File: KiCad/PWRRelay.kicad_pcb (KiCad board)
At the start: 2 copper layers, 46.4 x 65.4 mm, 19 parts, among them J0 Conn_01x02, K1 SANYOU_SRD_Form_C, Q1 IRLML2060, Q2 IRLML2060, U1 MOC3063M, X2 Conn_01x03_Male

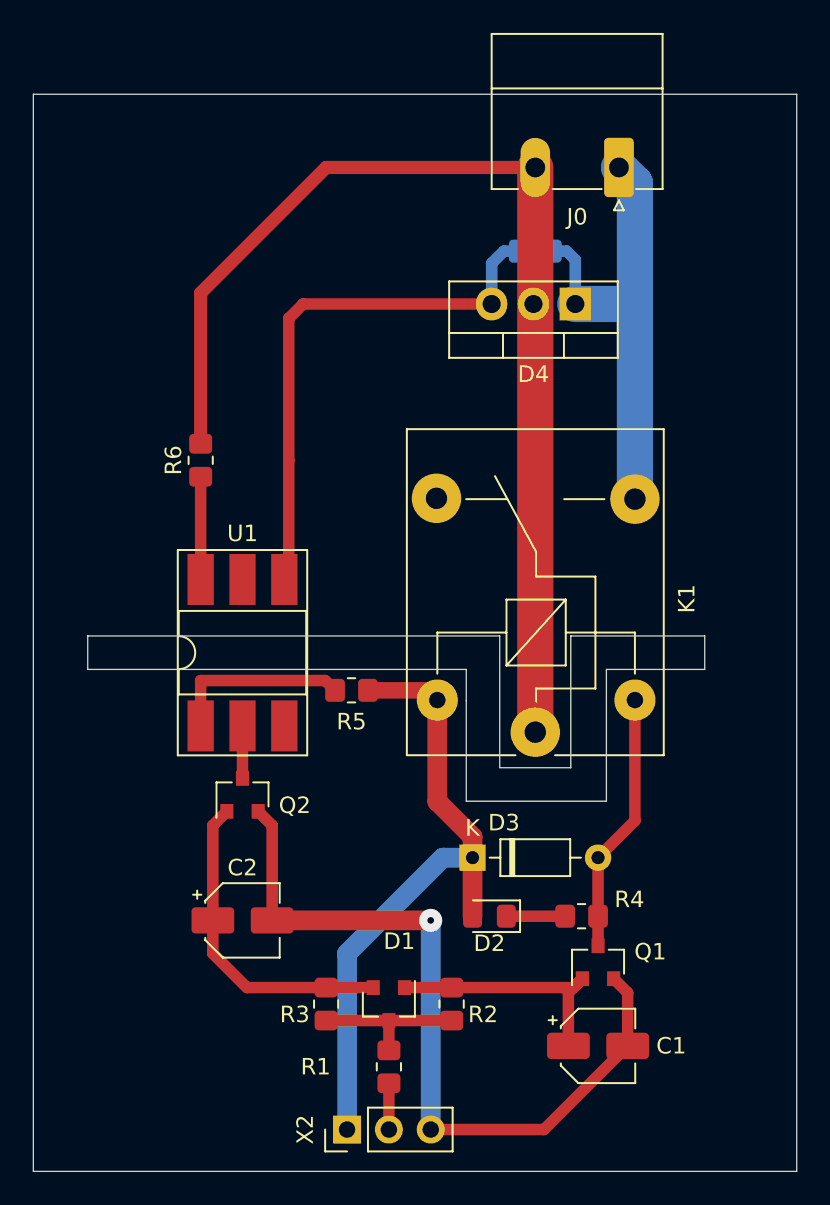
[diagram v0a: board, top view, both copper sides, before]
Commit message: Rework
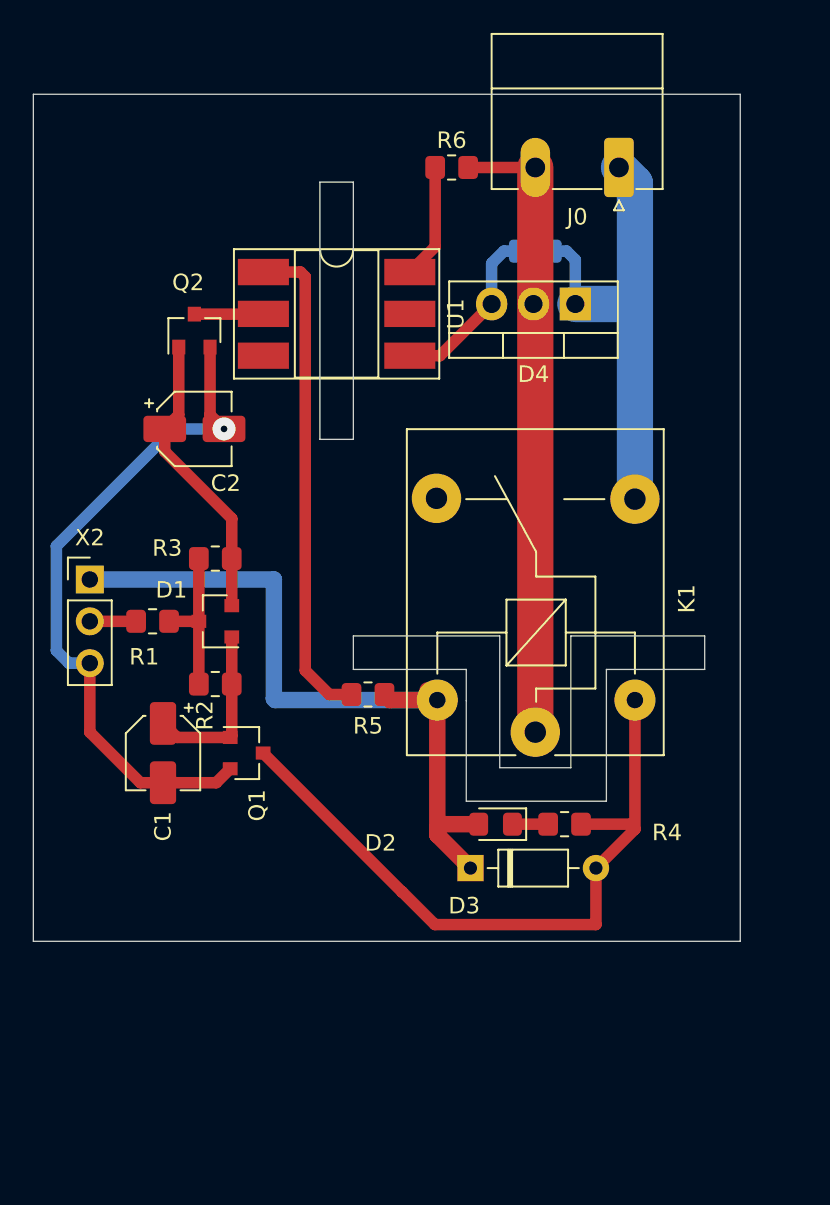
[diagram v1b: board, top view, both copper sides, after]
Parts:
- moved X2 36.9 mm to (33.9, 54.2), turned to 0 degrees
- moved C1 31.8 mm to (38.4, 64.8), turned to 270 degrees
- moved R1 30.6 mm to (37.7, 56.8), turned to 0 degrees
- moved C2 30.0 mm to (40.3, 45.1)
- moved Q2 28.3 mm to (40.3, 39.1)
- moved R3 27.9 mm to (41.5, 53.0), turned to 0 degrees
- moved D1 25.5 mm to (41.5, 56.8), turned to 180 degrees
- moved Q1 24.8 mm to (43.4, 64.8), turned to 0 degrees
- moved R2 24.2 mm to (41.5, 60.6), turned to 0 degrees
- moved R6 23.4 mm to (55.9, 29.2), turned to 0 degrees
- moved U1 21.4 mm to (48.9, 38.1), turned to 0 degrees
- moved R4 5.68 mm to (62.7, 69.1)
- moved D2 5.60 mm to (58.5, 69.1)
- moved R5 1.03 mm to (50.8, 61.2)
- moved D3 0.65 mm to (57.0, 71.8)
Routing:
- net /PWR_220_0: track 66.9 -> 38.4 mm
- net Net-(D3-Pad2): track 15.8 -> 42.5 mm
- net /PWR_220_LOW_1: track 33.1 -> 10.7 mm
- net Net-(R5-Pad2): track 11.2 -> 30.5 mm
- net VCC: track 39.2 -> 46.2 mm
- net GND: track 47.8 -> 41.5 mm
- net Net-(C1-Pad1): track 15.5 -> 10.6 mm
- net Net-(C2-Pad1): track 19.6 -> 17.7 mm
- net Net-(D2-Pad1): track 3.57 -> 2.17 mm
- net Net-(Q2-Pad3): track 3.19 -> 4.20 mm
- net /PWR_220_LOW_0: track 6.24 -> 6.99 mm
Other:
- board size 46.4 x 65.4 mm -> 42.9 x 51.4 mm
